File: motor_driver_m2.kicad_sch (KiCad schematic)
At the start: 33 parts, among them J7 Conn_01x01_Pin, J8 Conn_01x01_Pin, J9 Conn_01x01_Pin, M2 DRV8320SRTVR, Q10 NP80N06D6, Q11 NP80N06D6, Q12 NP80N06D6, Q7 NP80N06D6, Q8 NP80N06D6, Q9 NP80N06D6

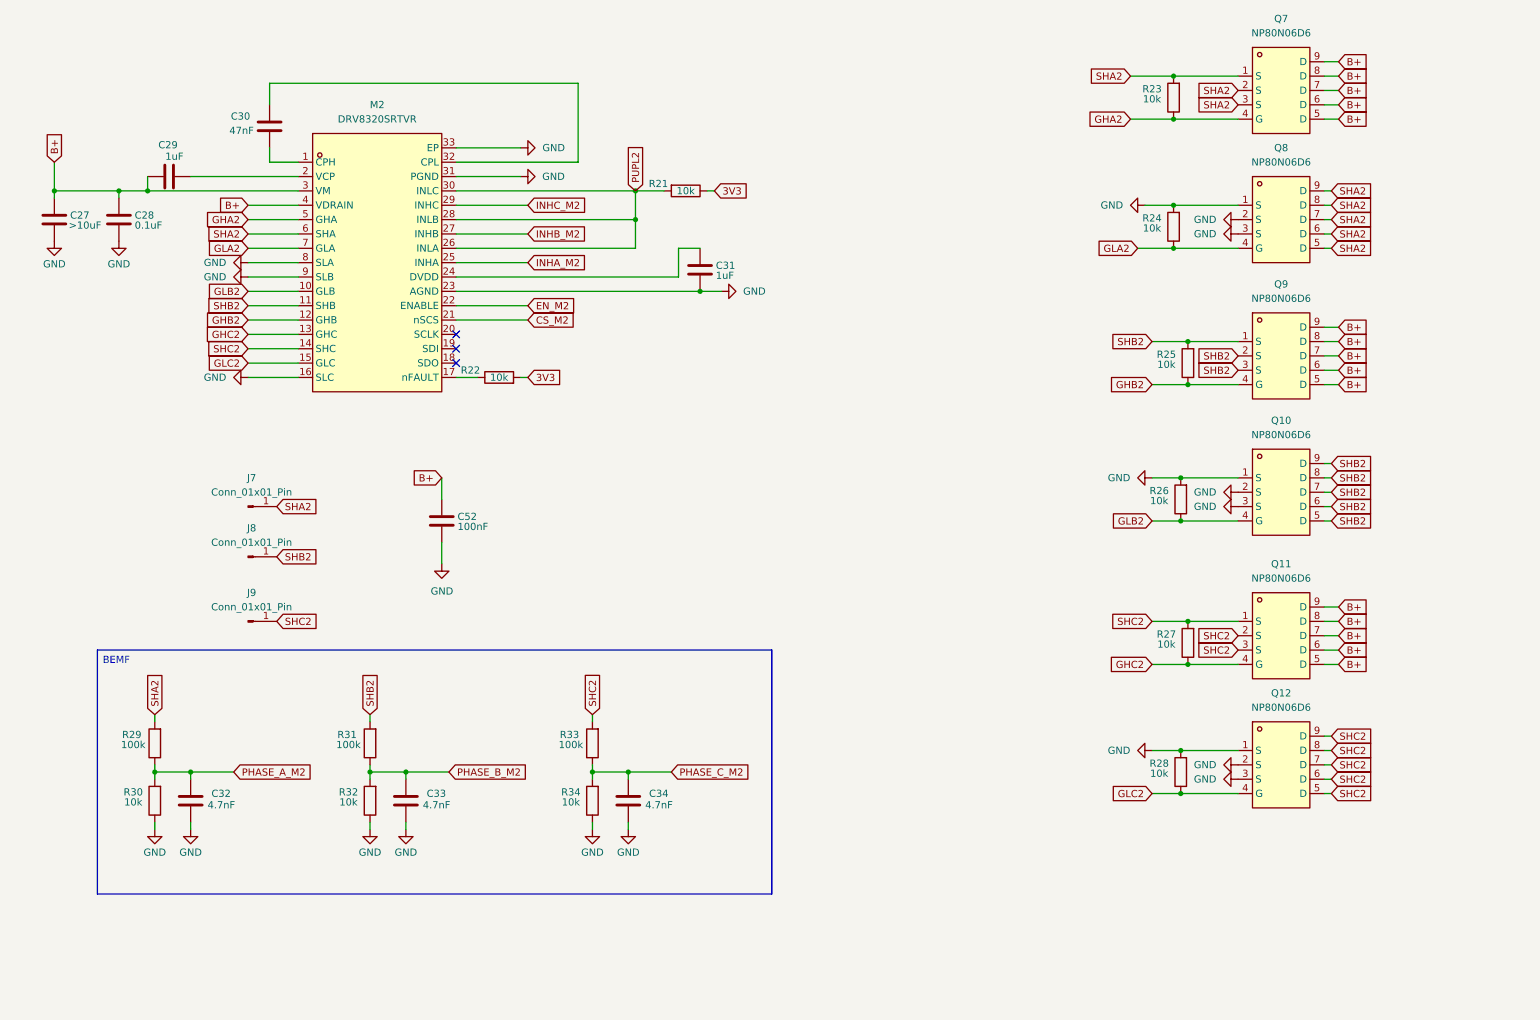
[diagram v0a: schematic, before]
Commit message: complete change in architecture,work in progress
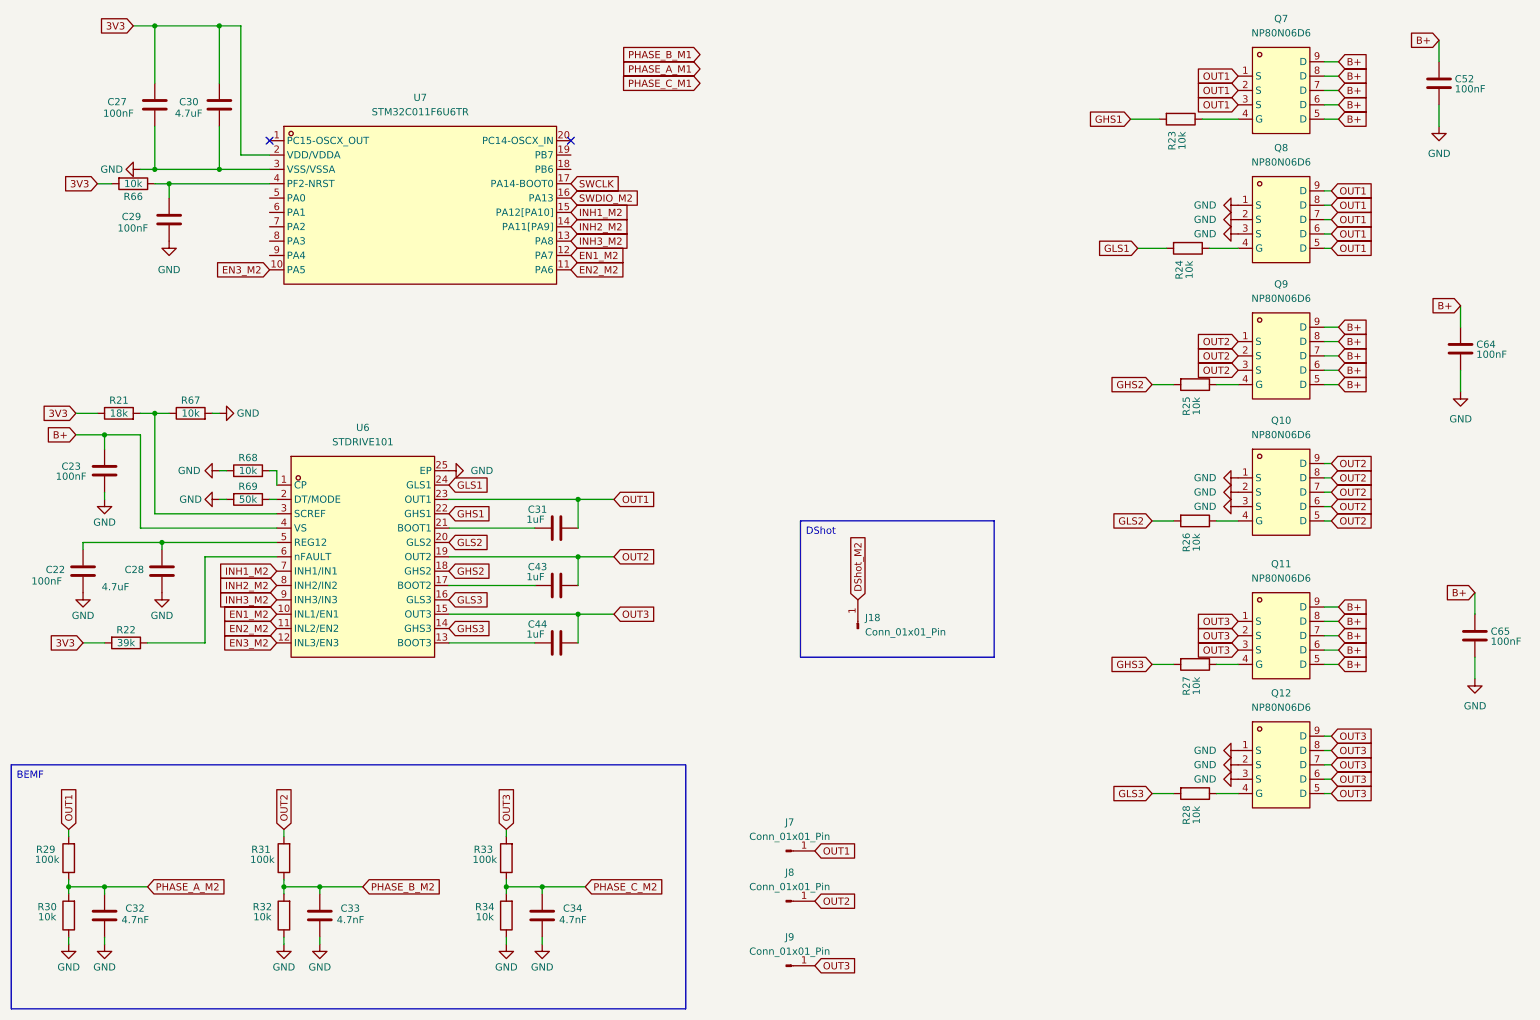
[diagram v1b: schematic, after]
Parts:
- removed M2: DRV8320SRTVR, easyeda2kicad:WQFN-32_L5.0-W5.0-P0.50-TL-EP3.5, symbol easyeda2kicad:DRV8320SRTVR
- added C22, C64, C65: 100nF, easyeda2kicad:C0603, symbol Device:C
- added C23: 100nF, easyeda2kicad:C0402, symbol Device:C
- added C43, C44: 1uF, easyeda2kicad:C0402, symbol Device:C
- added J18: Conn_01x01_Pin, deshan:Conn_1x1_small, symbol Connector:Conn_01x01_Pin
- added R66, R67, R68: 10k, easyeda2kicad:R0402, symbol Device:R
- added R69: 50k, easyeda2kicad:R0402, symbol Device:R
- added U6: STDRIVE101, easyeda2kicad:QFN-24_L4.0-W4.0-P0.50-BL-EP2.7, symbol easyeda2kicad:STDRIVE101
- added U7: STM32C011F6U6TR, easyeda2kicad:UFQFPN-20_L3.0-W3.0-P0.50-TL, symbol easyeda2kicad:STM32C011F6U6TR
- C27: value >10uF -> 100nF; footprint easyeda2kicad:C0603 -> easyeda2kicad:C0402
- C28: value 0.1uF -> 4.7uF; footprint easyeda2kicad:C0402 -> easyeda2kicad:C0603
- C29: value 1uF -> 100nF; footprint easyeda2kicad:C0603 -> easyeda2kicad:C0402
- C30: value 47nF -> 4.7uF; footprint easyeda2kicad:C0603 -> easyeda2kicad:C0402
- C31: footprint easyeda2kicad:C0603 -> easyeda2kicad:C0402
- R21: value 10k -> 18k
- R22: value 10k -> 39k
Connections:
- net 3V3: now also C27.1, C30.1, R66.2, U7.2 (VDD/VDDA)
- net B+: now also C23.1, C64.1, C65.1, U6.4 (VS); no longer C27.1, C28.1, C29.1
- net GND: now also C29.2, C30.2, C22.2, C23.2, C64.2, C65.2, R67.2, R68.1, R69.2, U6.25 (EP), U7.3 (VSS/VSSA); no longer C31.2, R24.2, R26.2, R28.2
- net at R22.1: now also U6.6 (nFAULT)
- net OUT1: now reaches C31.1
- net OUT1: now also J7.1 (Pin_1), Q7.1 (S), Q7.2 (S), Q7.3 (S), Q8.5 (D), Q8.6 (D), Q8.7 (D), Q8.8 (D), Q8.9 (D), R29.2, U6.23 (OUT1)
- net GHA2: no longer names the net of Q7.4 (G), R23.1
- net GHB2: no longer names the net of Q9.4 (G), R25.1
- net GHC2: no longer names the net of Q11.4 (G), R27.1
- net GLA2: no longer names the net of Q8.4 (G), R24.1
- net GLB2: no longer names the net of Q10.4 (G), R26.1
- net GLC2: no longer names the net of Q12.4 (G), R28.1
- net PUPL2: no longer names the net of R21.2
- net PUPL2: now also R67.1, U6.3 (SCREF)
- removed net SHA2: J7.1 (Pin_1), Q7.1 (S), Q7.2 (S), Q7.3 (S), Q8.5 (D), Q8.6 (D), Q8.7 (D), Q8.8 (D), Q8.9 (D), R23.2, R29.2
- net SHB2 renamed OUT2
- net OUT2: now also C43.1, U6.19 (OUT2); no longer R25.2
- net SHC2 renamed OUT3
- net OUT3: now also C44.1, U6.15 (OUT3); no longer R27.2
- new net: C31.2, U6.21 (BOOT1)
- new net: R68.2, U6.1 (CP)
- new net: C29.1, R66.1, U7.4 (PF2-NRST)
- new net: C43.2, U6.17 (BOOT2)
- new net: C22.1, C28.1, U6.5 (REG12)
- new net: C44.2, U6.13 (BOOT3)
- new net: R69.1, U6.2 (DT/MODE)
- new net DShot_M2: J18.1 (Pin_1)
- new net EN1_M2: U6.10 (INL1/EN1), U7.12 (PA7)
- new net EN2_M2: U6.11 (INL2/EN2), U7.11 (PA6)
- new net EN3_M2: U6.12 (INL3/EN3), U7.10 (PA5)
- new net GHS1: R23.2, U6.22 (GHS1)
- new net GHS2: R25.2, U6.18 (GHS2)
- new net GHS3: R27.2, U6.14 (GHS3)
- new net GLS1: R24.2, U6.24 (GLS1)
- new net GLS2: R26.2, U6.20 (GLS2)
- new net GLS3: R28.2, U6.16 (GLS3)
- new net INH1_M2: U6.7 (INH1/IN1), U7.15 (PA12[PA10])
- new net INH2_M2: U6.8 (INH2/IN2), U7.14 (PA11[PA9])
- new net INH3_M2: U6.9 (INH3/IN3), U7.13 (PA8)
- new net SWCLK: U7.17 (PA14-BOOT0)
- new net SWDIO_M2: U7.16 (PA13)
- no-connect marks 3 -> 2
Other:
- moved on the sheet: C32, C33, C34, C52, J7, J8, J9, R23, R24, R25, R26, R27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
